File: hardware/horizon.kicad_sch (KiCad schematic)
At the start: 8 parts, among them J1 USB_C_Receptacle_PowerOnly_6P, SW1 SW_Push, U1 ESP32-S3, U2 NCP1529A

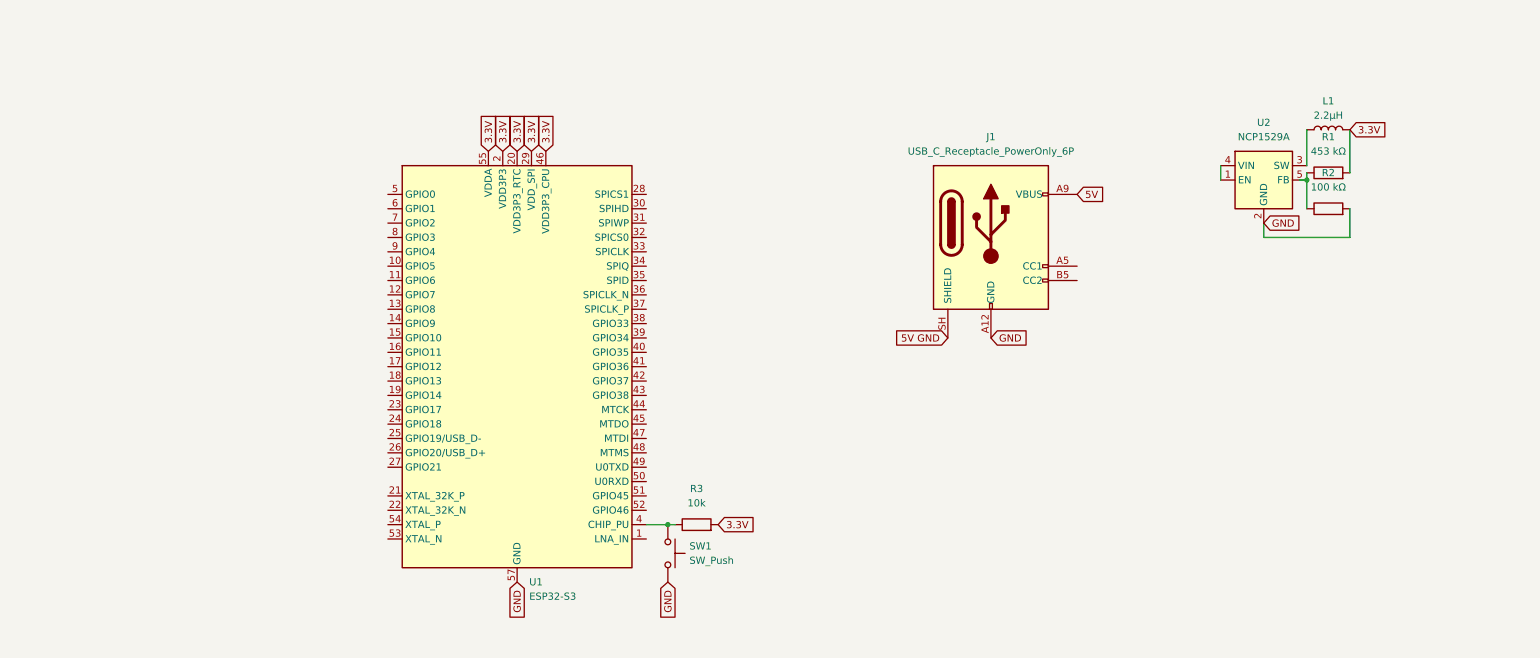
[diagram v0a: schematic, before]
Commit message: Working on PD and QSPI
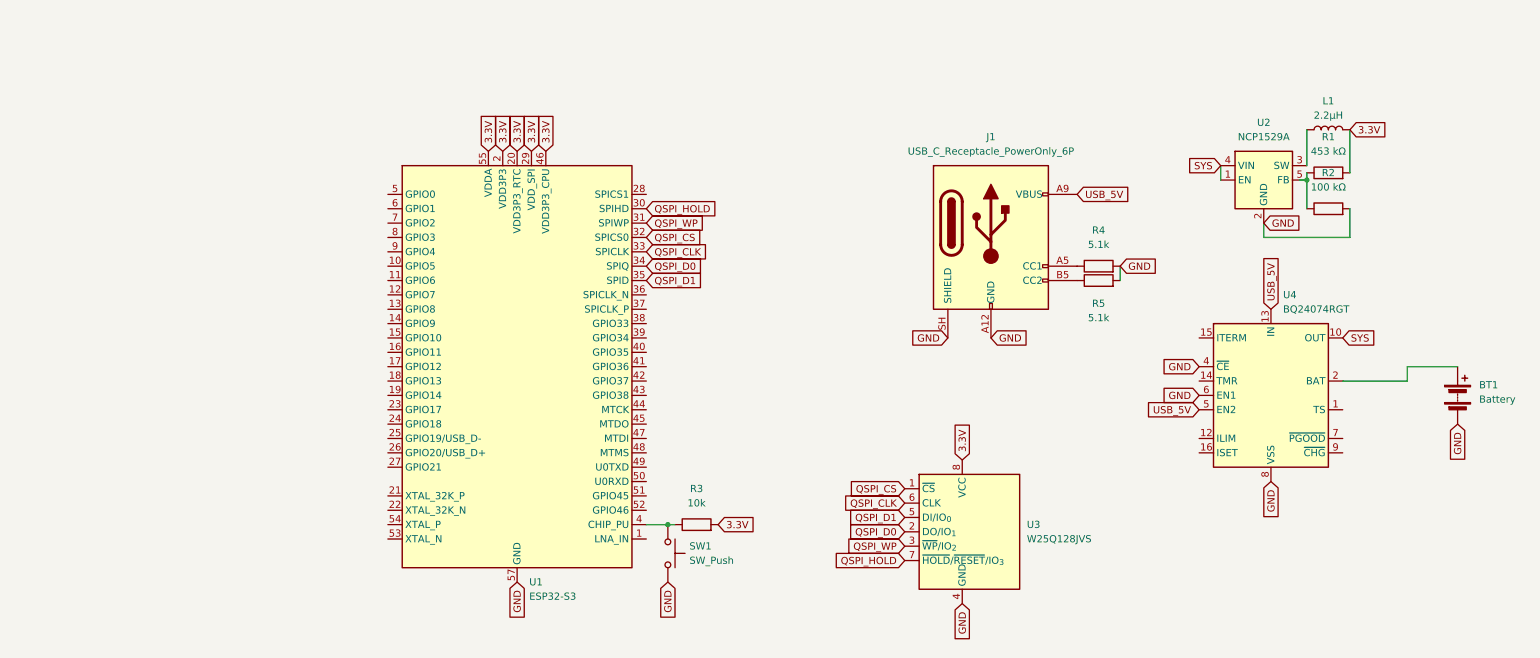
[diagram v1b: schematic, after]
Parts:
- added BT1: Battery, symbol Device:Battery
- added R4, R5: 5.1k, symbol Device:R
- added U3: W25Q128JVS, Package_SO:SOIC-8_5.3x5.3mm_P1.27mm, symbol Memory_Flash:W25Q128JVS
- added U4: BQ24074RGT, Package_DFN_QFN:VQFN-16-1EP_3x3mm_P0.5mm_EP1.6x1.6mm, symbol Battery_Management:BQ24074RGT
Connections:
- net 5V GND is gone; now on net GND: J1.SH (SHIELD)
- net 3.3V: now also U3.8 (VCC)
- net GND: now also BT1.2 (-), R4.2, R5.2, U3.4 (GND), U4.17 (VSS), U4.4 (~{CE}), U4.6 (EN1), U4.8 (VSS)
- net at J1.A5 (CC1): now also R4.1
- net at J1.B5 (CC2): now also R5.1
- net QSPI_HOLD: now reaches U1.30 (SPIHD)
- net QSPI_HOLD: now also U3.7 (~{HOLD}/~{RESET}/IO_{3})
- net QSPI_WP: now reaches U1.31 (SPIWP)
- net QSPI_WP: now also U3.3 (~{WP}/IO_{2})
- net QSPI_CS: now reaches U1.32 (SPICS0)
- net QSPI_CS: now also U3.1 (~{CS})
- net QSPI_CLK: now reaches U1.33 (SPICLK)
- net QSPI_CLK: now also U3.6 (CLK)
- net QSPI_D0: now reaches U1.34 (SPIQ)
- net QSPI_D0: now also U3.2 (DO/IO_{1})
- net QSPI_D1: now reaches U1.35 (SPID)
- net QSPI_D1: now also U3.5 (DI/IO_{0})
- net SYS: now reaches U2.1 (EN), U2.4 (VIN)
- net SYS: now also U4.10 (OUT), U4.11 (OUT)
- net 5V renamed USB_5V
- net USB_5V: now also U4.13 (IN), U4.5 (EN2)
- new net: BT1.1 (+), U4.2 (BAT), U4.3 (BAT)

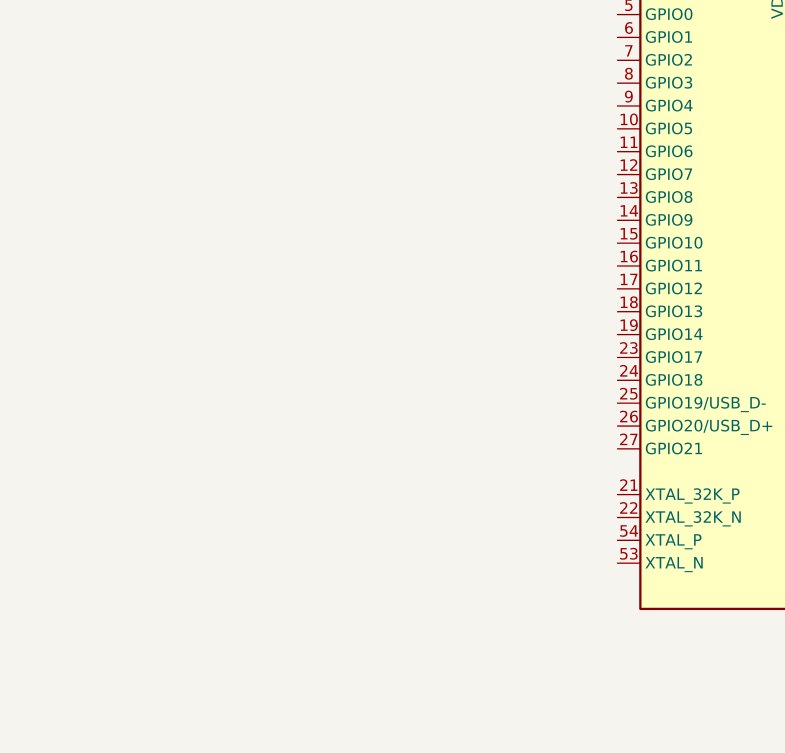
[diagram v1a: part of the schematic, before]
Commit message: Working on schematic
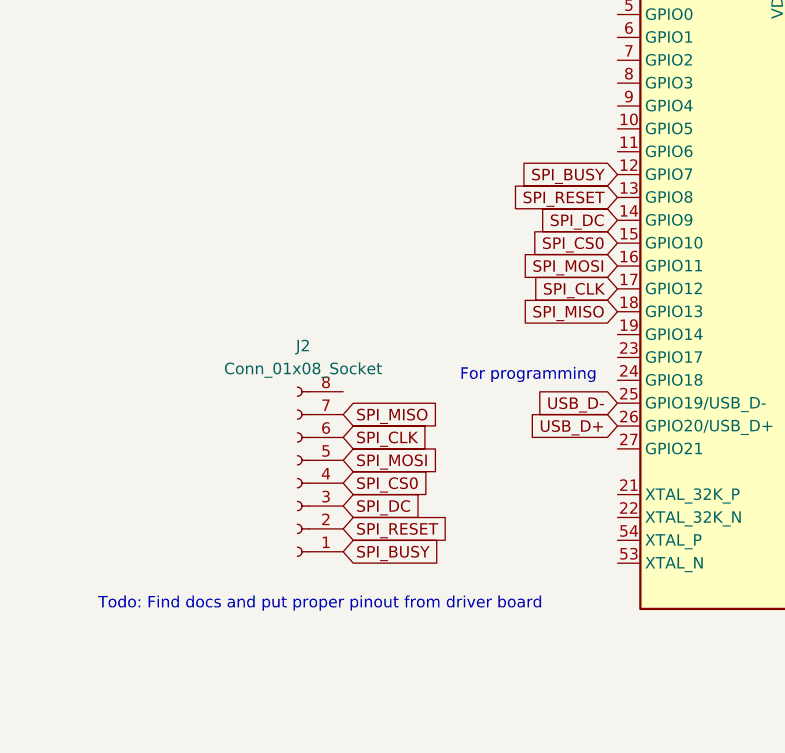
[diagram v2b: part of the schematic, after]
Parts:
- added J2: Conn_01x08_Socket, symbol Connector:Conn_01x08_Socket
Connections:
- net SPI_BUSY: now reaches U1.12 (GPIO7)
- net SPI_BUSY: now also J2.1 (Pin_1)
- net SPI_RESET: now reaches U1.13 (GPIO8)
- net SPI_RESET: now also J2.2 (Pin_2)
- net SPI_DC: now reaches U1.14 (GPIO9)
- net SPI_DC: now also J2.3 (Pin_3)
- net SPI_CS0: now reaches U1.15 (GPIO10)
- net SPI_CS0: now also J2.4 (Pin_4)
- net SPI_MOSI: now reaches U1.16 (GPIO11)
- net SPI_MOSI: now also J2.5 (Pin_5)
- net SPI_CLK: now reaches U1.17 (GPIO12)
- net SPI_CLK: now also J2.6 (Pin_6)
- net SPI_MISO: now reaches U1.18 (GPIO13)
- net SPI_MISO: now also J2.7 (Pin_7)
- net USB_D-: now reaches U1.25 (GPIO19/USB_D-)
- net USB_D+: now reaches U1.26 (GPIO20/USB_D+)
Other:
- note added: "For programming"
- note added: "Todo: Find docs and put proper pinout from driver board"

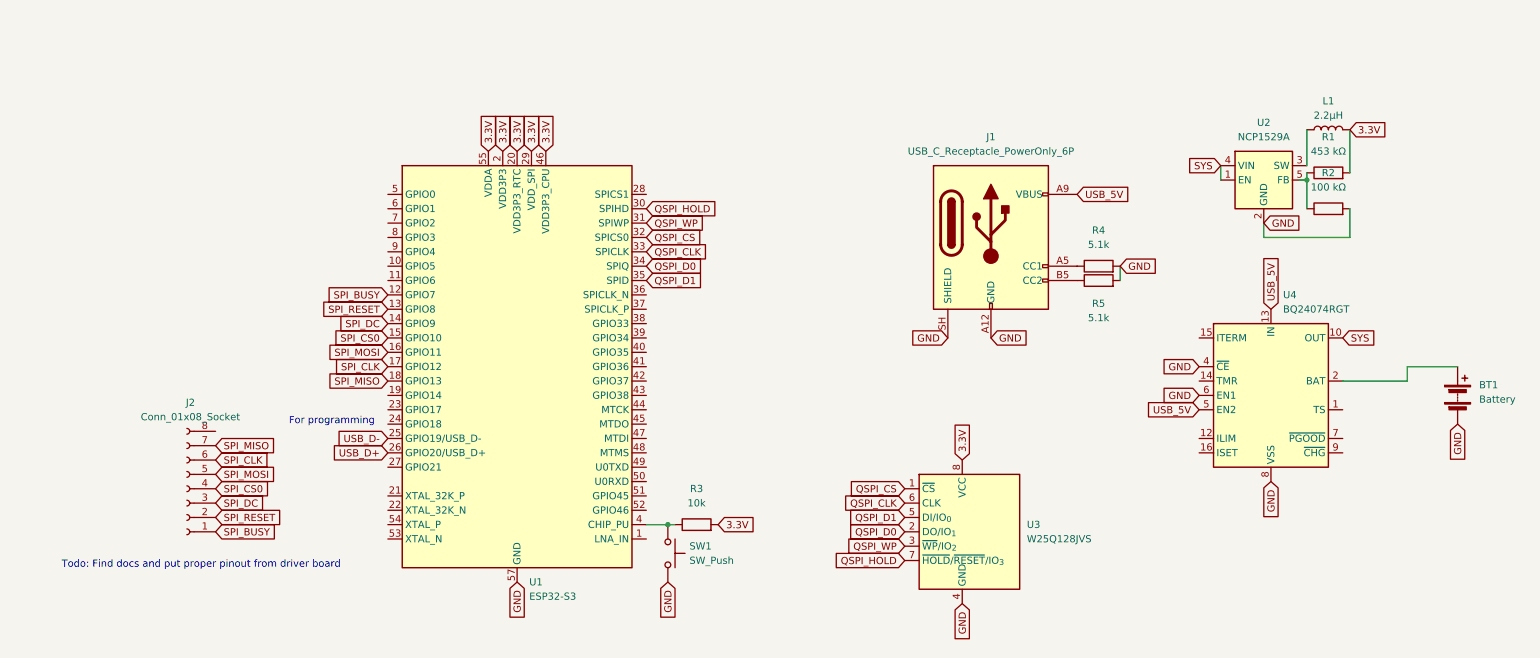
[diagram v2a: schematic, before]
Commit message: Finished schematic draft
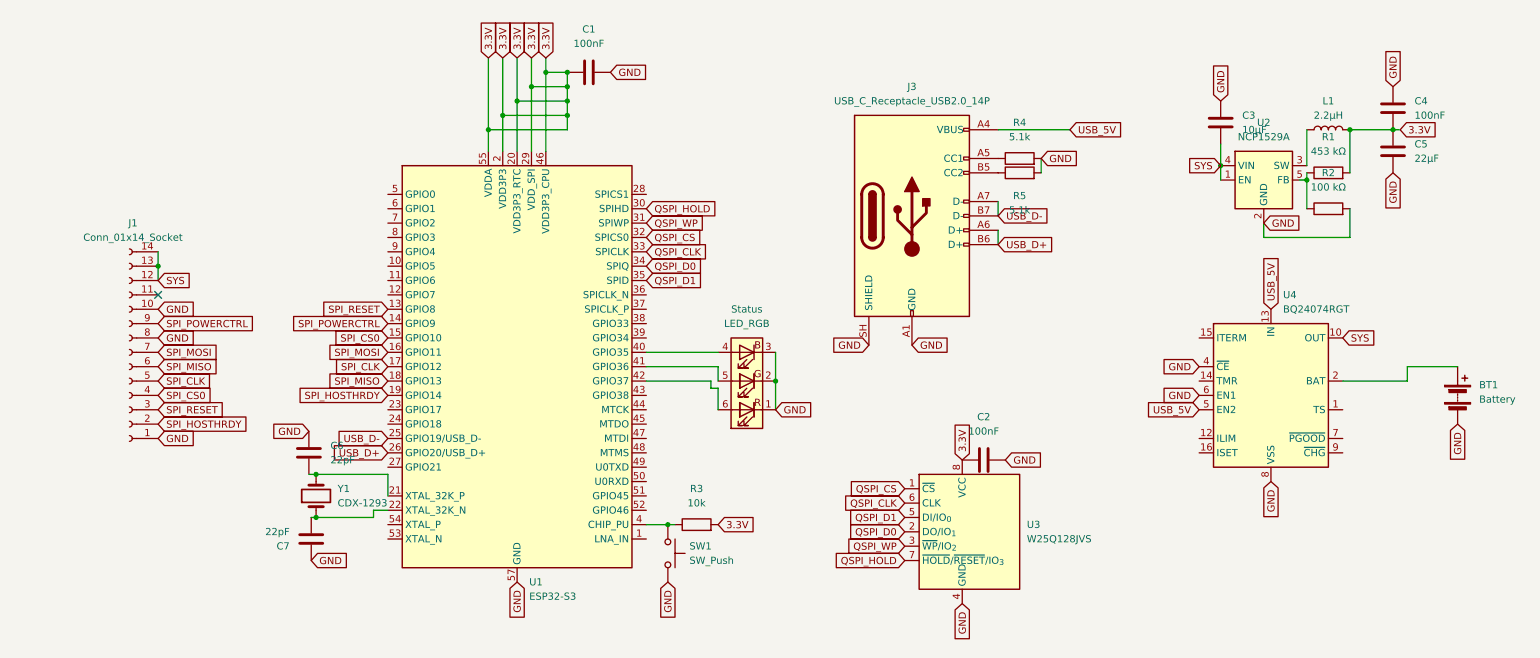
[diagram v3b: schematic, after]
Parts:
- removed J1: USB_C_Receptacle_PowerOnly_6P, symbol Connector:USB_C_Receptacle_PowerOnly_6P
- removed J2: Conn_01x08_Socket, symbol Connector:Conn_01x08_Socket
- added C1, C2, C4: 100nF, symbol Device:C
- added C3: 10µF, symbol Device:C
- added C5: 22µF, symbol Device:C
- added C6, C7: 22pF, symbol Device:C
- added J1: Conn_01x14_Socket, symbol Connector:Conn_01x14_Socket
- added J3: USB_C_Receptacle_USB2.0_14P, symbol Connector:USB_C_Receptacle_USB2.0_14P
- added Status: LED_RGB, symbol Device:LED_RGB
- added Y1: CDX-1293, symbol Device:Crystal
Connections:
- net 3.3V: now also C1.1, C2.1, C4.1, C5.1
- net GND: now also C1.2, C2.2, C3.2, C4.2, C5.2, C6.2, C7.2, J1.1 (Pin_1), J1.10 (Pin_10), J1.8 (Pin_8), J3.A1 (GND), J3.A12 (GND), J3.B1 (GND), J3.B12 (GND), J3.SH (SHIELD), Status.1 (RK), Status.2 (GK), Status.3 (BK)
- net SPI_CLK: now also J1.5 (Pin_5)
- net SPI_CS0: now also J1.4 (Pin_4)
- net SPI_MISO: now also J1.6 (Pin_6)
- net SPI_MOSI: now also J1.7 (Pin_7)
- net SPI_RESET: now also J1.3 (Pin_3)
- net SYS: now also C3.1, J1.12 (Pin_12), J1.13 (Pin_13), J1.14 (Pin_14)
- net USB_5V: now also J3.A4 (VBUS), J3.A9 (VBUS), J3.B4 (VBUS), J3.B9 (VBUS)
- net USB_D+: now also J3.A6 (D+), J3.B6 (D+)
- net USB_D-: now also J3.A7 (D-), J3.B7 (D-)
- net at R5.1: now also J3.B5 (CC2)
- net at R4.1: now also J3.A5 (CC1)
- net SPI_HOSTHRDY: now reaches U1.19 (GPIO14)
- net SPI_HOSTHRDY: now also J1.2 (Pin_2)
- net at U1.21 (XTAL_32K_P): now also C6.1, Y1.2
- net at U1.22 (XTAL_32K_N): now also C7.1, Y1.1
- net at U1.40 (GPIO35): now also Status.4 (BA)
- net at U1.41 (GPIO36): now also Status.5 (GA)
- net at U1.42 (GPIO37): now also Status.6 (RA)
- net SPI_BUSY: no longer names the net of U1.12 (GPIO7)
- net SPI_DC renamed SPI_POWERCTRL
- net SPI_POWERCTRL: now also J1.9 (Pin_9)
- no-connect marks 0 -> 1
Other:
- note removed: "For programming"
- note removed: "Todo: Find docs and put proper pinout from driver board"
